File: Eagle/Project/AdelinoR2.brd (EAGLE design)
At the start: 47 x 53.3 mm, 79 parts, among them J1 DC-044-A, J2 YELLOW-8P-2.54, J3 YELLOW-6P-2.54, J4 YELLOW-8P-2.54, J5 YELLOW-8P-2.54, J6 4P-2.0, J7 YELLOW-2X3P-2.54, J8 4P-2.0, Q1 NCE3407A, Q2 CJ2305, SW1 TS-1101F, U1 CJT1117-3.3-SOT223, U2 MP1496DJ-SOT23-8, U3 ESP-12F / OPL: 317060163 / SM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, U4 ATMEGA32U4-MUR-QFN44, U5 ATMEGA32U4-TQFP44, X1 306010049_XTAL_16MHZ-3225_4P

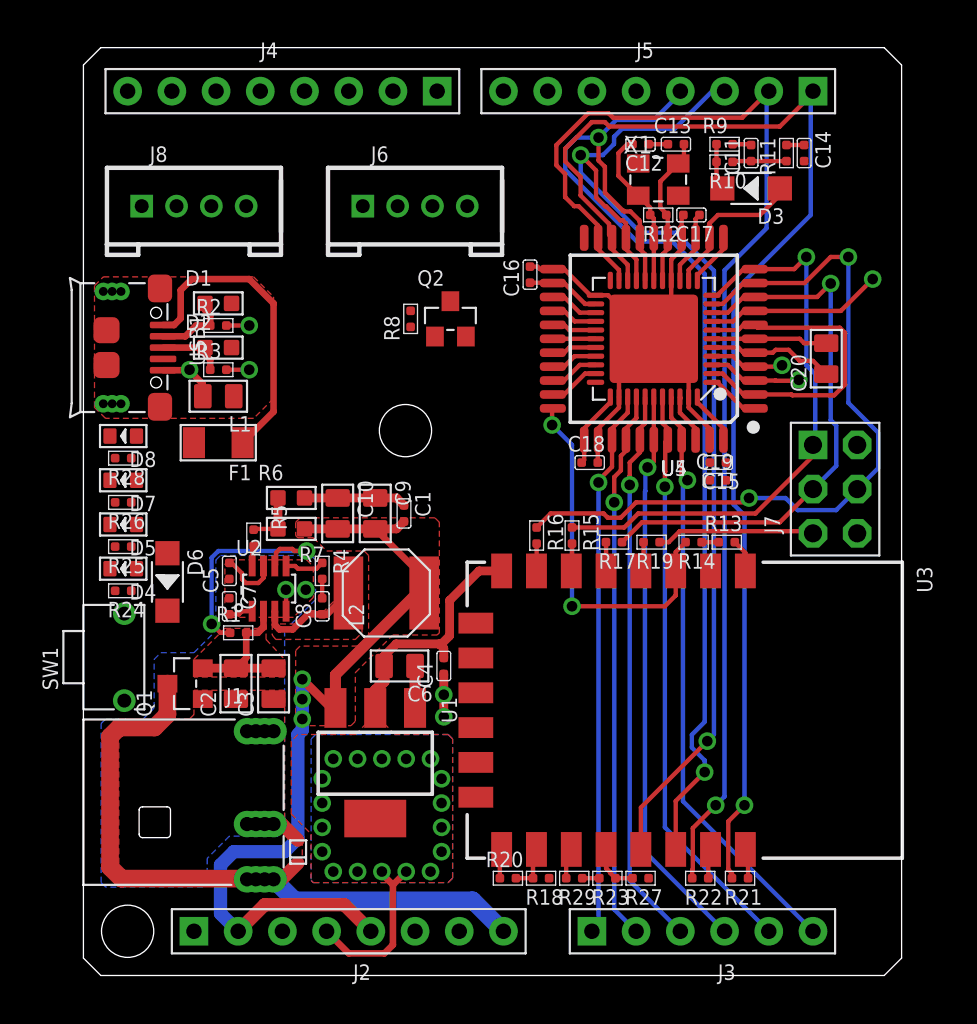
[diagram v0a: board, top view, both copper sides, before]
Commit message: Routing wip.
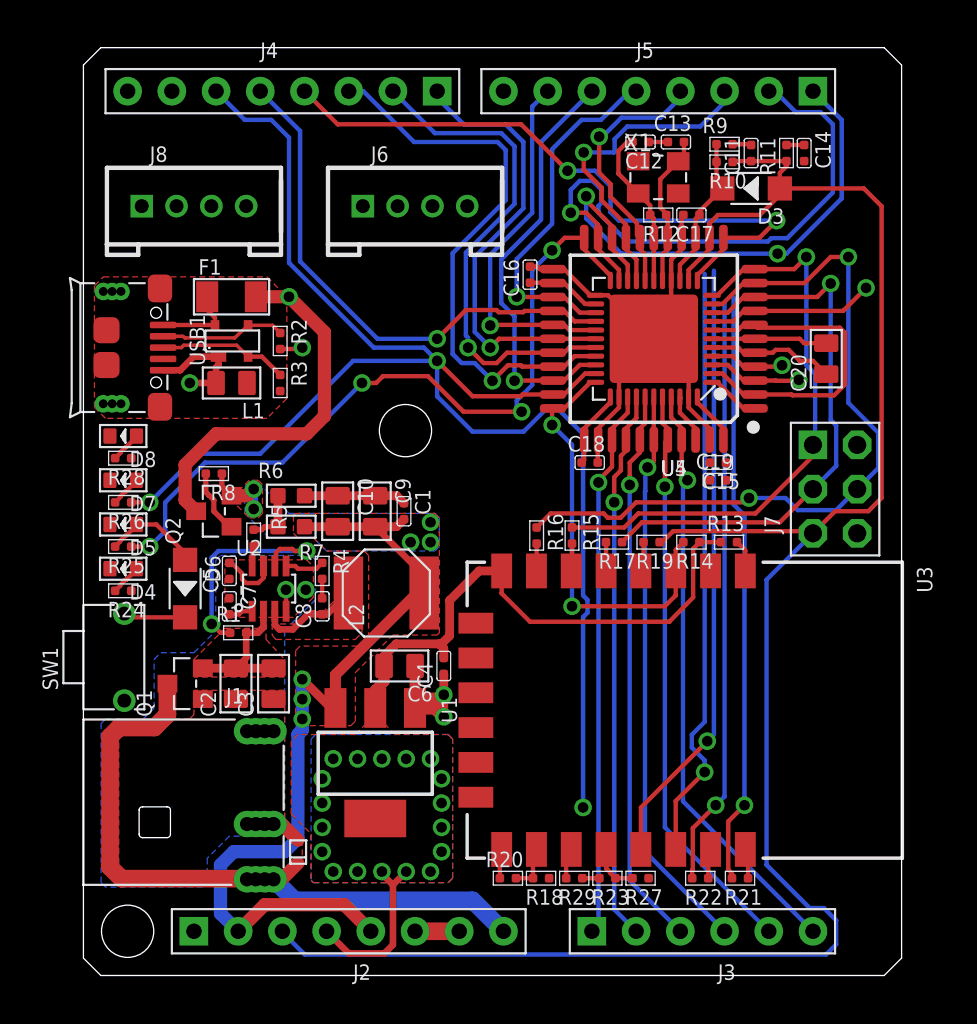
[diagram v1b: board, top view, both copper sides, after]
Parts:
- removed D1, D2: 1K 1/10W, Seeed-Fuse:D0603
- added ESD1: PRTR5V0U2X, Seeed-OPL-2017-01-Diode-james:SOT-143B
- moved Q2 17.5 mm to (7.49, 26.7), turned to 90 degrees
- moved R8 14.4 mm to (7.49, 28.8), turned to 270 degrees
- moved F1 8.42 mm to (8.51, 39.0), turned to 0 degrees
- moved R2 3.67 mm to (11.3, 36.4), turned to 0 degrees
- moved R3 3.64 mm to (11.3, 34.0), turned to 0 degrees
- moved D6 1.09 mm to (5.84, 22.2)
- moved L1 1.08 mm to (8.51, 34.0)
- moved C1 0.13 mm to (18.4, 26.7)
- moved C10 0.13 mm to (14.6, 26.7)
- moved C9 0.13 mm to (16.8, 26.7)
- moved R13 0.13 mm to (37.1, 24.9)
- moved R14 0.13 mm to (34.9, 24.9)
- moved R6 0.13 mm to (11.9, 27.6)
- moved X1 0.13 mm to (33.0, 45.8)
- moved R7 0.13 mm to (11.9, 25.8)
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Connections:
- net GND: no longer D1.1, D2.1
- net N$1: now also ESD1.3; no longer D1.2
- net N$2: now also ESD1.2; no longer D2.2
- net N$9: now also ESD1.4
- net UGND: now also ESD1.1
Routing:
- net RESET: track 21.1 -> 110.1 mm
- net PIN_D13: track 2.95 -> 88.8 mm, vias 0 -> 3
- net ACT_LED: track 0.00 -> 43.7 mm, vias 0 -> 4
- net PIN_D11: track 3.07 -> 37.6 mm, vias 0 -> 2
- net PIN_D10: track 2.70 -> 32.9 mm, vias 0 -> 1
- net PIN_D12: track 2.70 -> 30.6 mm, vias 0 -> 1
- net PIN_D9: track 2.57 -> 29.1 mm, vias 0 -> 1
- net PIN_D8: track 2.45 -> 26.0 mm, vias 0 -> 1
- net VUSB: track 19.3 -> 41.0 mm, vias 0 -> 1
- net PIN_D5: track 2.82 -> 24.1 mm, vias 0 -> 1
- net PIN_D6: track 2.57 -> 21.0 mm, vias 0 -> 1
- net PIN_D4: track 2.82 -> 20.4 mm, vias 0 -> 1
- net +3V3: track 26.1 -> 43.2 mm
- net PIN_D3: track 63.7 -> 49.7 mm
- net N$9: track 17.7 -> 4.82 mm
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- added copper zone on layer 16, net +5V
